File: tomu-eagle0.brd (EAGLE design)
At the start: 14.2 x 10.2 mm, 18 parts, among them U1 EFM32HG309F64G

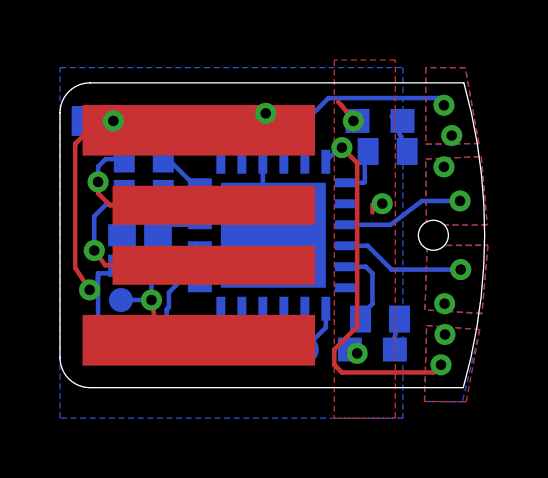
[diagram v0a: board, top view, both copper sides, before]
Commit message: still dealing with QFN 4x4 -> 5x5 issues
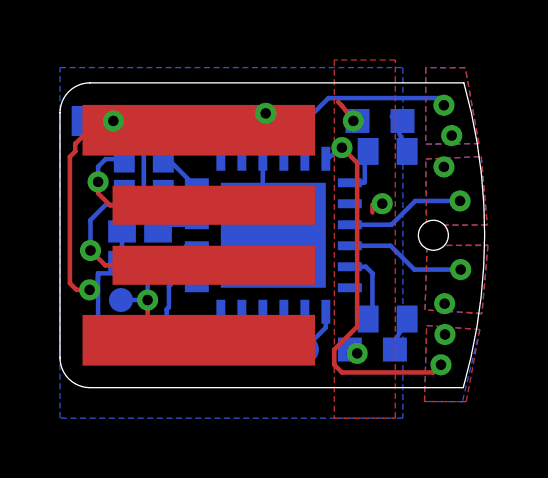
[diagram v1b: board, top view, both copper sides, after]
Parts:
- moved R2 0.25 mm to (10.9, 3.05)
- moved C2 0.13 mm to (2.67, 5.97)
- moved C3 0.13 mm to (2.67, 4.95)
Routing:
- net +3V3: track 3.95 -> 6.88 mm
- net GND: track 27.0 -> 27.6 mm
